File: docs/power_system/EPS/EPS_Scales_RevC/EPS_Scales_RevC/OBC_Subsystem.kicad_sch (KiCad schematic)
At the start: 28 parts, among them U10 INA230

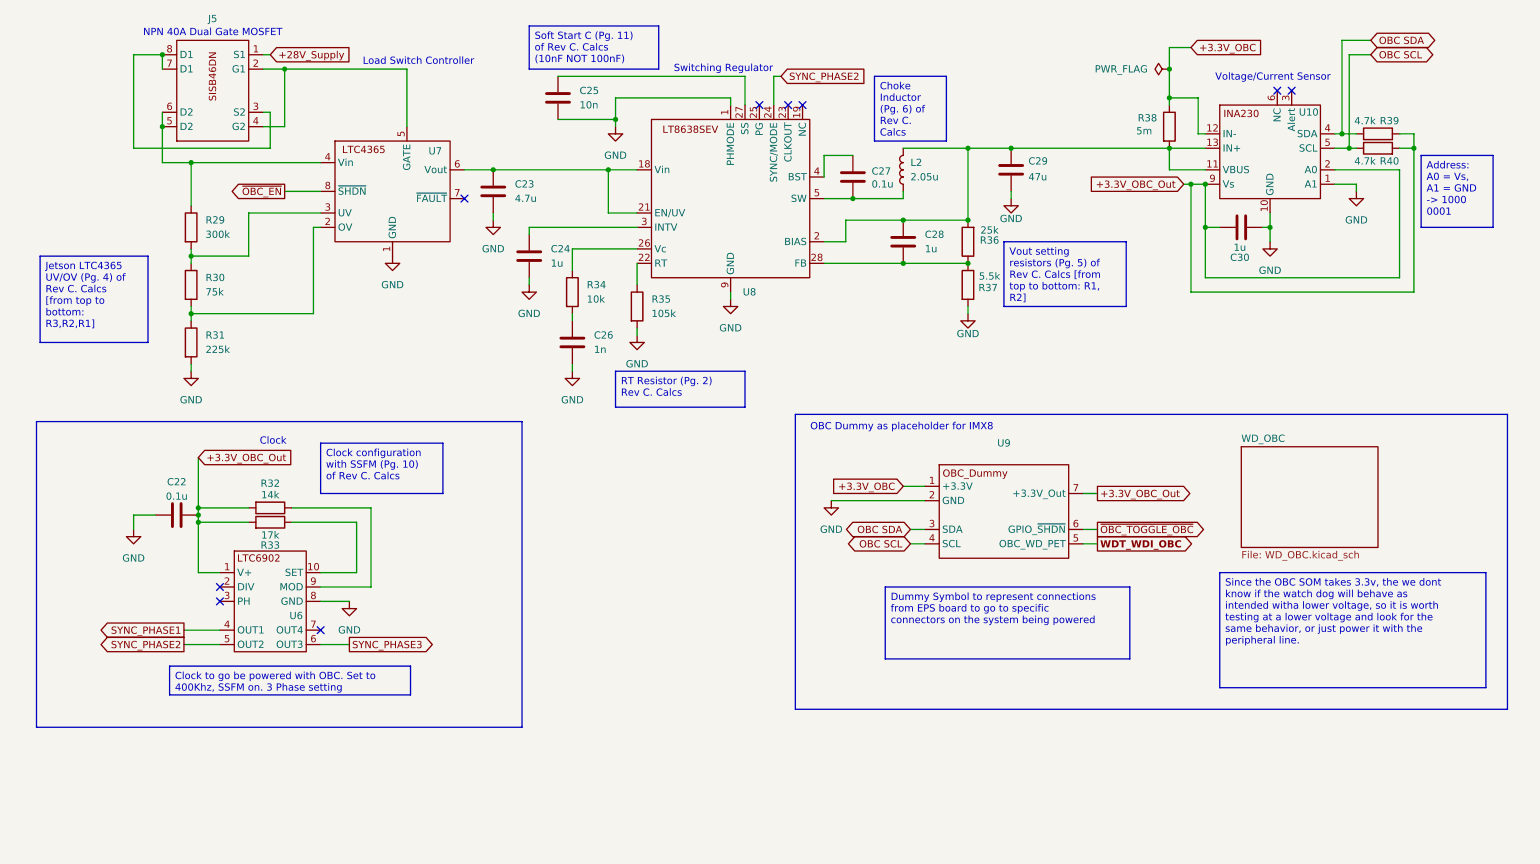
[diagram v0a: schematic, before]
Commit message: Layout Revisions
Organizing components and layering considerations
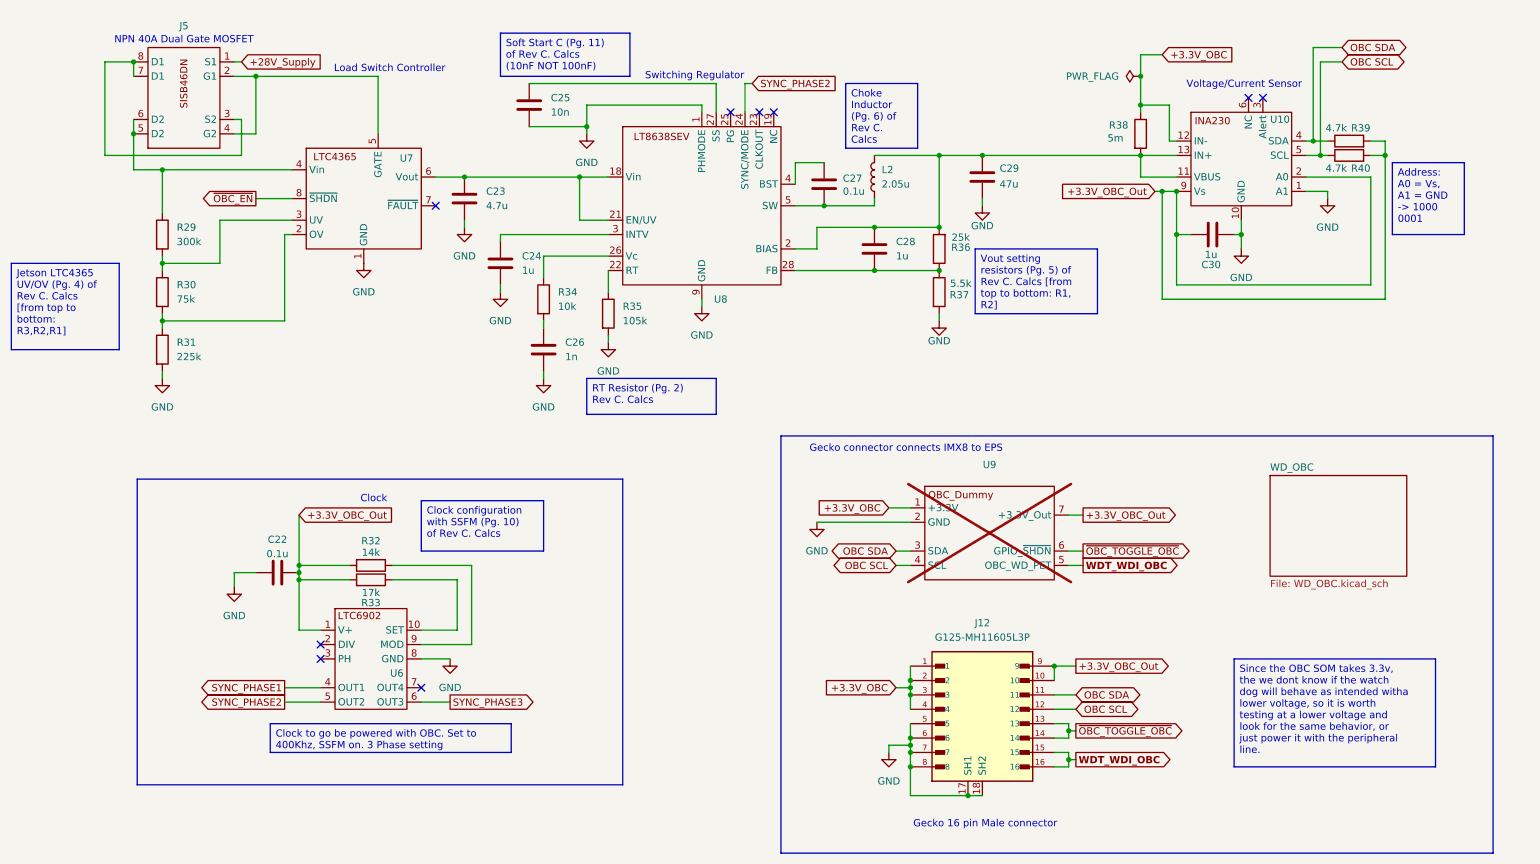
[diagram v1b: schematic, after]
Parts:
- added J12: G125-MH11605L3P, RevC Footprints:HARWIN_G125-MH11605L3P, symbol 16 Pin Gecko Male Connector:G125-MH11605L3P
- U9: now not fitted; now left out of the parts list
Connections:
- net +3.3V_OBC: now also J12.1, J12.2, J12.3, J12.4
- net +3.3V_OBC_Out: now also J12.10, J12.9
- net GND: now also J12.17 (SH1), J12.18 (SH2), J12.5, J12.6, J12.7, J12.8
- net OBC SCL: now also J12.12
- net OBC SDA: now also J12.11
- net WDT_WDI_OBC: now also J12.15, J12.16
- net ~{OBC_TOGGLE_OBC}: now also J12.13, J12.14
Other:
- note added: "Gecko 16 pin Male connector"
- note added: "Gecko connector connects IMX8 to EPS"
- note removed: "OBC Dummy as placeholder for IMX8"
- moved on the sheet: C22, C23, C24, C25, C26, C27, C28, C29, C30, J5, L2, R29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
